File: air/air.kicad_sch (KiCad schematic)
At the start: 8 parts, among them CN1 SM06B-GHS-TB(LF)(SN), U1 3SP-H2S-50_110-304, U2 SCD41-D-R2, U3 ADS1115IDGS

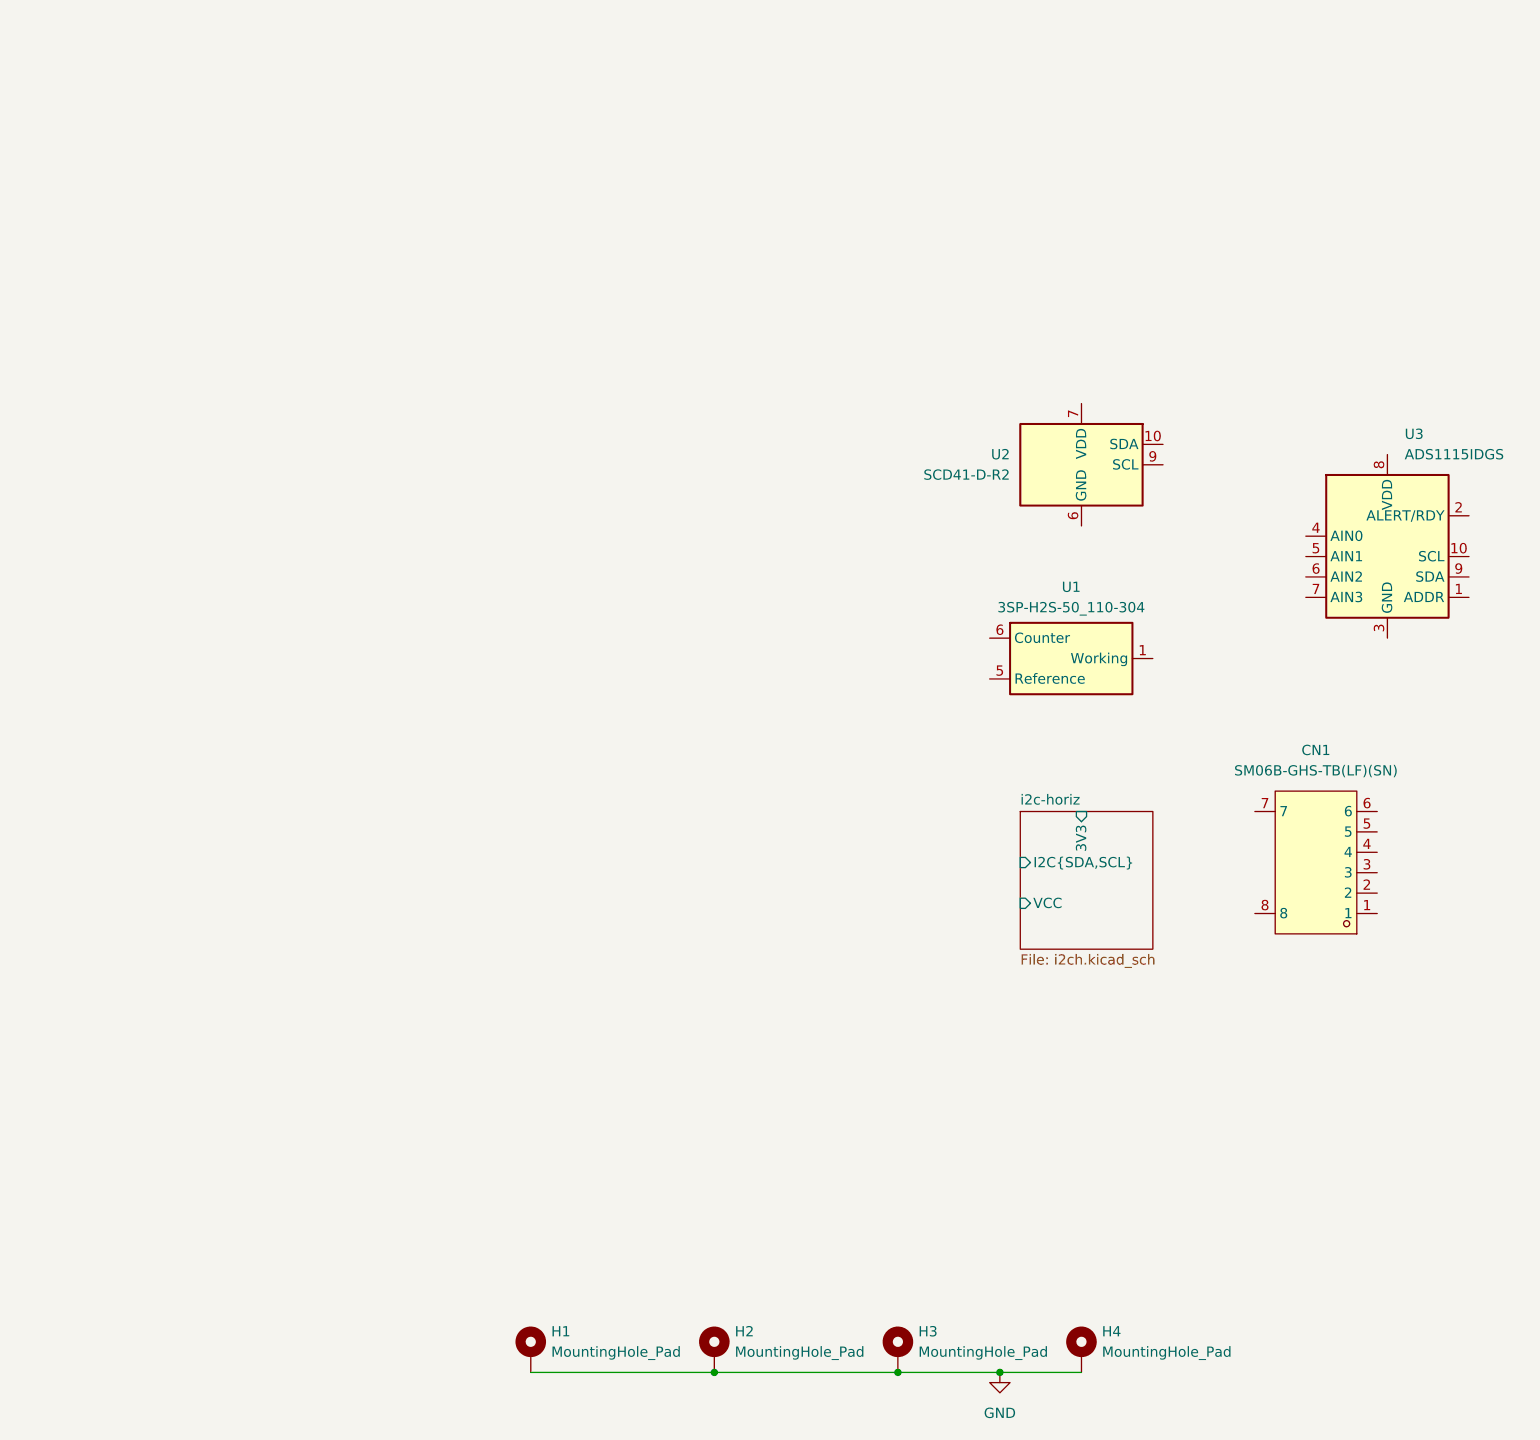
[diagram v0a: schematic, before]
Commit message: first version of air sensor
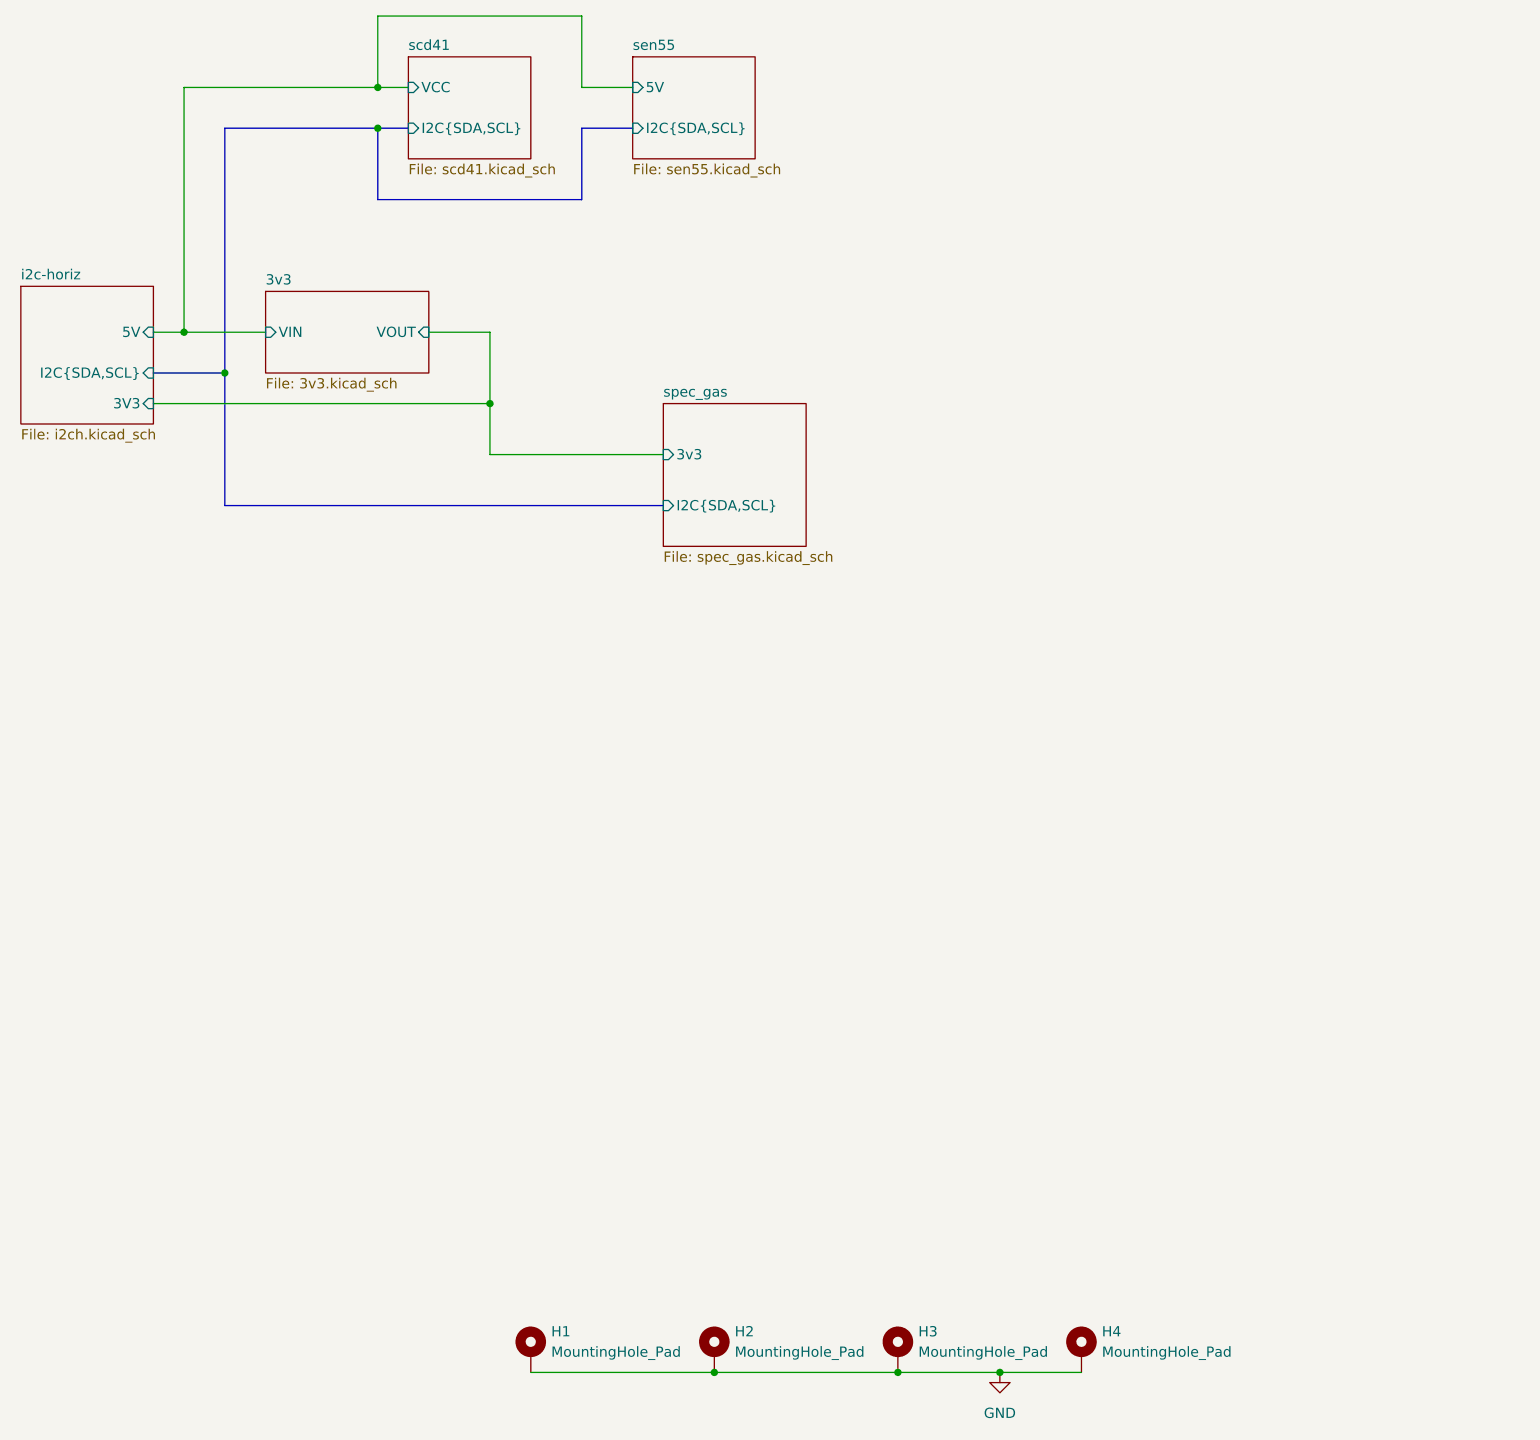
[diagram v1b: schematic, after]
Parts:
- removed CN1: SM06B-GHS-TB(LF)(SN), easyeda2kicad:CONN-TH_SM06B-GHS-TB-LF-SN, symbol easyeda2kicad:SM06B-GHS-TB(LF)(SN)
- removed U1: 3SP-H2S-50_110-304, Sensor:SPEC_110-xxx_SMD-10Pin_20x20mm_P4.0mm, symbol Sensor_Gas:3SP-H2S-50_110-304
- removed U2: SCD41-D-R2, Sensor:Sensirion_SCD4x-1EP_10.1x10.1mm_P1.25mm_EP4.8x4.8mm, symbol Sensor_Gas:SCD41-D-R2
- removed U3: ADS1115IDGS, Package_SO:TSSOP-10_3x3mm_P0.5mm, symbol Analog_ADC:ADS1115IDGS
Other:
- added sheet 3v3 (3v3.kicad_sch)
- added sheet scd41 (scd41.kicad_sch)
- added sheet sen55 (sen55.kicad_sch)
- added sheet spec_gas (spec_gas.kicad_sch)
- sheet i2c-horiz ports: added 5V; removed VCC
